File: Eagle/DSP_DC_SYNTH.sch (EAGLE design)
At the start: 83 parts, among them J16 U.FL_CONN, J17 U.FL_CONN, J2 3.5HEADPHONEJACK, J5 U.FL_CONN, J6 U.FL_CONN, U1 5V_REG, U2 MIXER, U3 DUAL_OP_AMP_LMV822, U4 DIGITAL_POTDIGITAL_POT, U5 TC1185-3.3VCT713, U6 LMX2326, U7 MAX2752, U8 RMK-3-93+

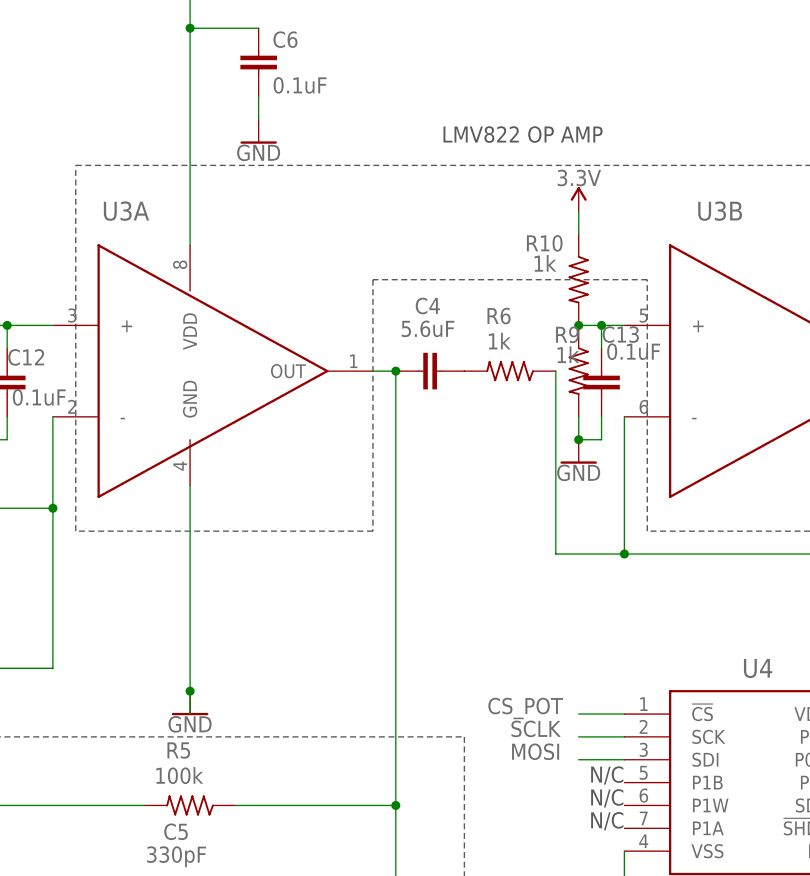
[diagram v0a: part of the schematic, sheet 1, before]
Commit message: started layout
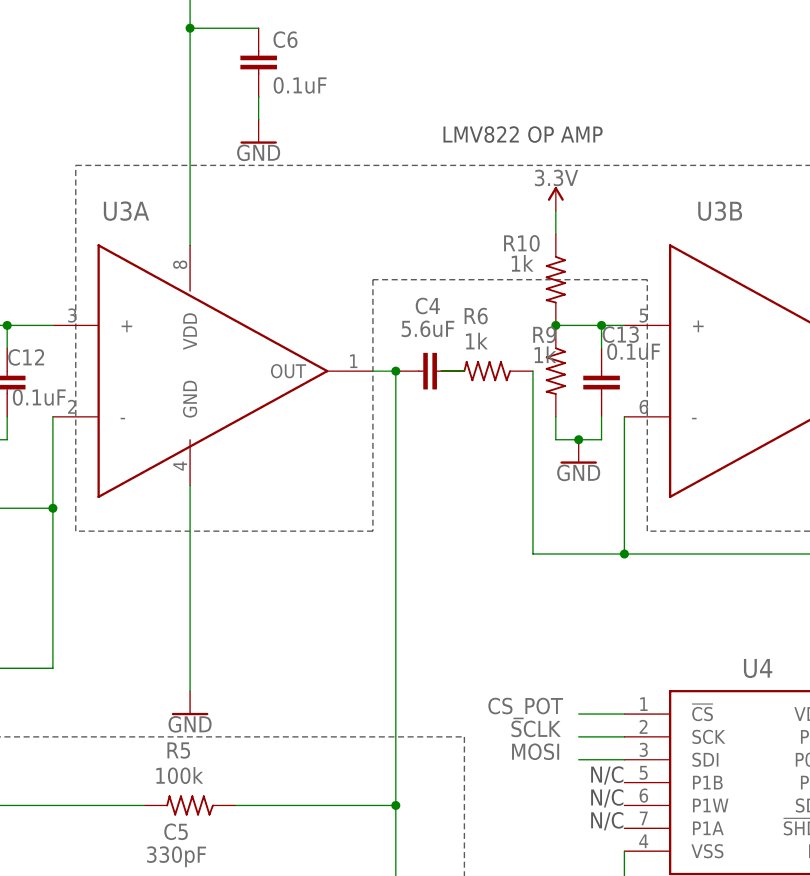
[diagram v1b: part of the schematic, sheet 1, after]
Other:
- moved on the sheet: R10, R6, R9
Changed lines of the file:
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@@
 <attribute name="VALUE" x="128.27" y="33.782" size="1.778" layer="96" align="center"/>
 </instance>
-<instance part="R6" gate="G$1" x="165.1" y="78.74" smashed="yes" rot="R180">
-<attribute name="NAME" x="163.83" y="84.8614" size="1.778" layer="95" align="center"/>
-<attribute name="VALUE" x="163.83" y="82.042" size="1.778" layer="96" align="center"/>
+<instance part="R6" gate="G$1" x="162.56" y="78.74" smashed="yes" rot="R180">
+<attribute name="NAME" x="161.29" y="84.8614" size="1.778" layer="95" align="center"/>
+<attribute name="VALUE" x="161.29" y="82.042" size="1.778" layer="96" align="center"/>
 </instance>
 <instance part="C4" gate="G$1" x="154.94" y="78.74" smashed="yes" rot="R90">
@@
 <attribute name="VALUE" x="104.14" y="99.314" size="1.778" layer="96" align="bottom-center"/>
 </instance>
-<instance part="R9" gate="G$1" x="172.72" y="78.74" smashed="yes" rot="R270">
-<attribute name="NAME" x="171.45" y="82.7786" size="1.778" layer="95" rot="R180" align="center"/>
-<attribute name="VALUE" x="171.45" y="80.518" size="1.778" layer="96" rot="R180" align="center"/>
-</instance>
-<instance part="R10" gate="G$1" x="172.72" y="88.9" smashed="yes" rot="R270">
-<attribute name="NAME" x="168.91" y="92.9386" size="1.778" layer="95" rot="R180" align="center"/>
-<attribute name="VALUE" x="168.91" y="90.678" size="1.778" layer="96" rot="R180" align="center"/>
-</instance>
-<instance part="SUPPLY6" gate="G$1" x="172.72" y="96.52" smashed="yes">
-<attribute name="VALUE" x="172.72" y="99.314" size="1.778" layer="96" align="bottom-center"/>
+<instance part="R9" gate="G$1" x="170.18" y="78.74" smashed="yes" rot="R270">
+<attribute name="NAME" x="168.91" y="82.7786" size="1.778" layer="95" rot="R180" align="center"/>
+<attribute name="VALUE" x="168.91" y="80.518" size="1.778" layer="96" rot="R180" align="center"/>
+</instance>
+<instance part="R10" gate="G$1" x="170.18" y="88.9" smashed="yes" rot="R270">
+<attribute name="NAME" x="166.37" y="92.9386" size="1.778" layer="95" rot="R180" align="center"/>
+<attribute name="VALUE" x="166.37" y="90.678" size="1.778" layer="96" rot="R180" align="center"/>
+</instance>
+<instance part="SUPPLY6" gate="G$1" x="170.18" y="96.52" smashed="yes">
+<attribute name="VALUE" x="170.18" y="99.314" size="1.778" layer="96" align="bottom-center"/>
 </instance>
 <instance part="GND17" gate="1" x="172.72" y="68.58" smashed="yes">
@@
 <wire x1="129.54" y1="66.04" x2="129.54" y2="43.18" width="0.1524" layer="91"/>
 <pinref part="GND9" gate="1" pin="GND"/>
-<wire x1="129.54" y1="43.18" x2="129.54" y2="40.64" width="0.1524" layer="91"/>
-<junction x="129.54" y="43.18"/>
 </segment>
 <segment>
@@
 </segment>
 <segment>
-<pinref part="R9" gate="G$1" pin="2"/>
 <pinref part="GND17" gate="1" pin="GND"/>
-<wire x1="172.72" y1="73.66" x2="172.72" y2="71.12" width="0.1524" layer="91"/>
 <wire x1="172.72" y1="71.12" x2="175.26" y2="71.12" width="0.1524" layer="91"/>
-<junction x="172.72" y="71.12"/>
 <pinref part="C13" gate="G$1" pin="2"/>
 <wire x1="175.26" y1="71.12" x2="175.26" y2="73.66" width="0.1524" layer="91"/>
+<pinref part="R9" gate="G$1" pin="2"/>
+<wire x1="170.18" y1="73.66" x2="170.18" y2="71.12" width="0.1524" layer="91"/>
+<wire x1="170.18" y1="71.12" x2="172.72" y2="71.12" width="0.1524" layer="91"/>
+<junction x="172.72" y="71.12"/>
 </segment>
 </net>
@@
 <pinref part="C4" gate="G$1" pin="2"/>
 <pinref part="R6" gate="G$1" pin="2"/>
+<wire x1="157.48" y1="78.74" x2="160.02" y2="78.74" width="0.1524" layer="91"/>
 </segment>
 </net>
@@
 <segment>
 <pinref part="U3" gate="B" pin="+"/>
-<wire x1="172.72" y1="83.82" x2="175.26" y2="83.82" width="0.1524" layer="91"/>
+<wire x1="170.18" y1="83.82" x2="175.26" y2="83.82" width="0.1524" layer="91"/>
 <pinref part="R10" gate="G$1" pin="2"/>
 <pinref part="R9" gate="G$1" pin="1"/>
-<junction x="172.72" y="83.82"/>
+<junction x="170.18" y="83.82"/>
 <pinref part="C13" gate="G$1" pin="1"/>
 <wire x1="175.26" y1="83.82" x2="177.8" y2="83.82" width="0.1524" layer="91"/>
@@
 <wire x1="223.52" y1="58.42" x2="177.8" y2="58.42" width="0.1524" layer="91"/>
 <pinref part="R6" gate="G$1" pin="1"/>
-<wire x1="177.8" y1="58.42" x2="170.18" y2="58.42" width="0.1524" layer="91"/>
-<wire x1="170.18" y1="78.74" x2="170.18" y2="58.42" width="0.1524" layer="91"/>
+<wire x1="177.8" y1="58.42" x2="167.64" y2="58.42" width="0.1524" layer="91"/>
+<wire x1="167.64" y1="78.74" x2="167.64" y2="58.42" width="0.1524" layer="91"/>
 <pinref part="U3" gate="B" pin="-"/>
 <wire x1="177.8" y1="73.66" x2="177.8" y2="58.42" width="0.1524" layer="91"/>
@@
 <pinref part="R10" gate="G$1" pin="1"/>
 <pinref part="SUPPLY6" gate="G$1" pin="3.3V"/>
-<wire x1="172.72" y1="93.98" x2="172.72" y2="96.52" width="0.1524" layer="91"/>
-</segment>
-<segment>
+<wire x1="170.18" y1="93.98" x2="170.18" y2="96.52" width="0.1524" layer="91"/>
+</segment>
+<segment>
